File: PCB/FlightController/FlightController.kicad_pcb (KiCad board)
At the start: 2 copper layers, 101.6 x 101.6 mm, 14 parts, among them J2 BATT IN, J3 BATT OUT, J4 BATT Reg IC, J5 Pump, J7 HallCircuit, Q1 P_CHANNEL, U1 XIAO-nRF52840-DIP, U2 RFM95W

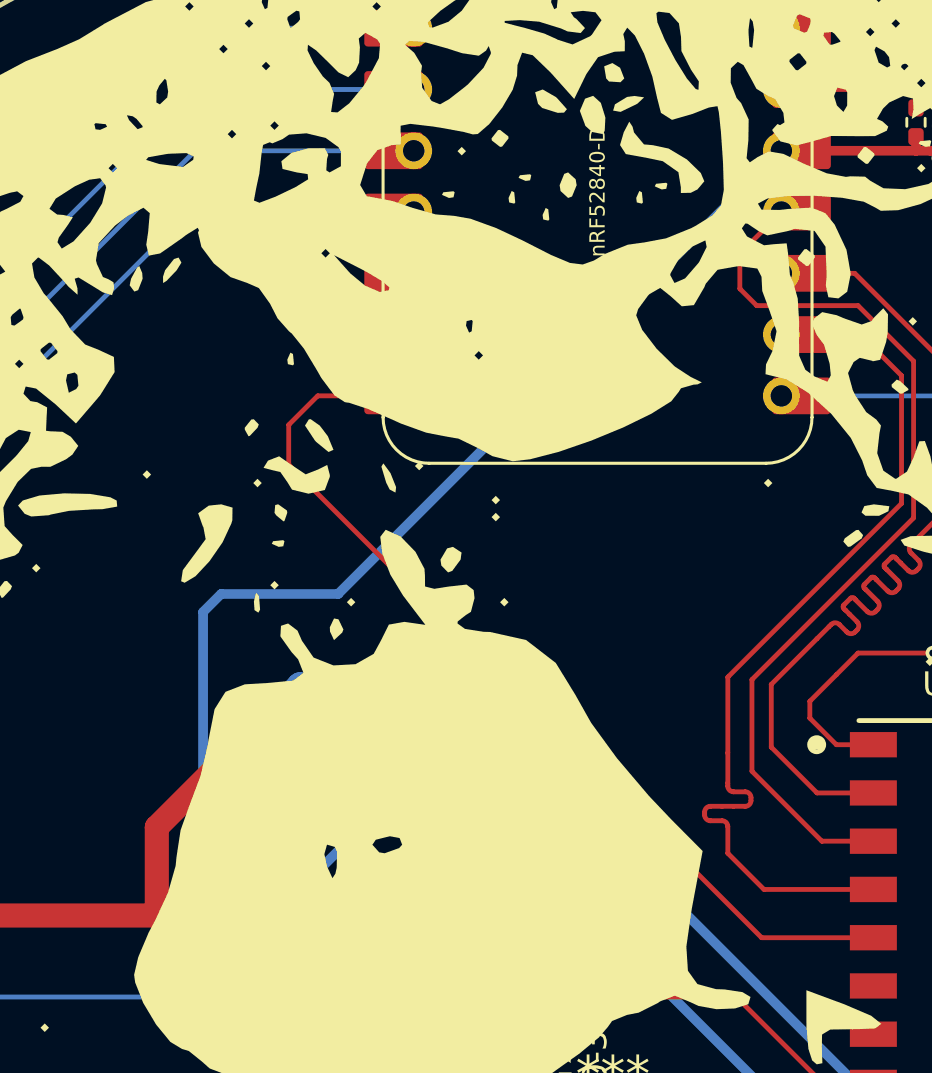
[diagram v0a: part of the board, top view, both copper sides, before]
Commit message: All boards should be finished. ACC otw, and an earlier version of the main board otw
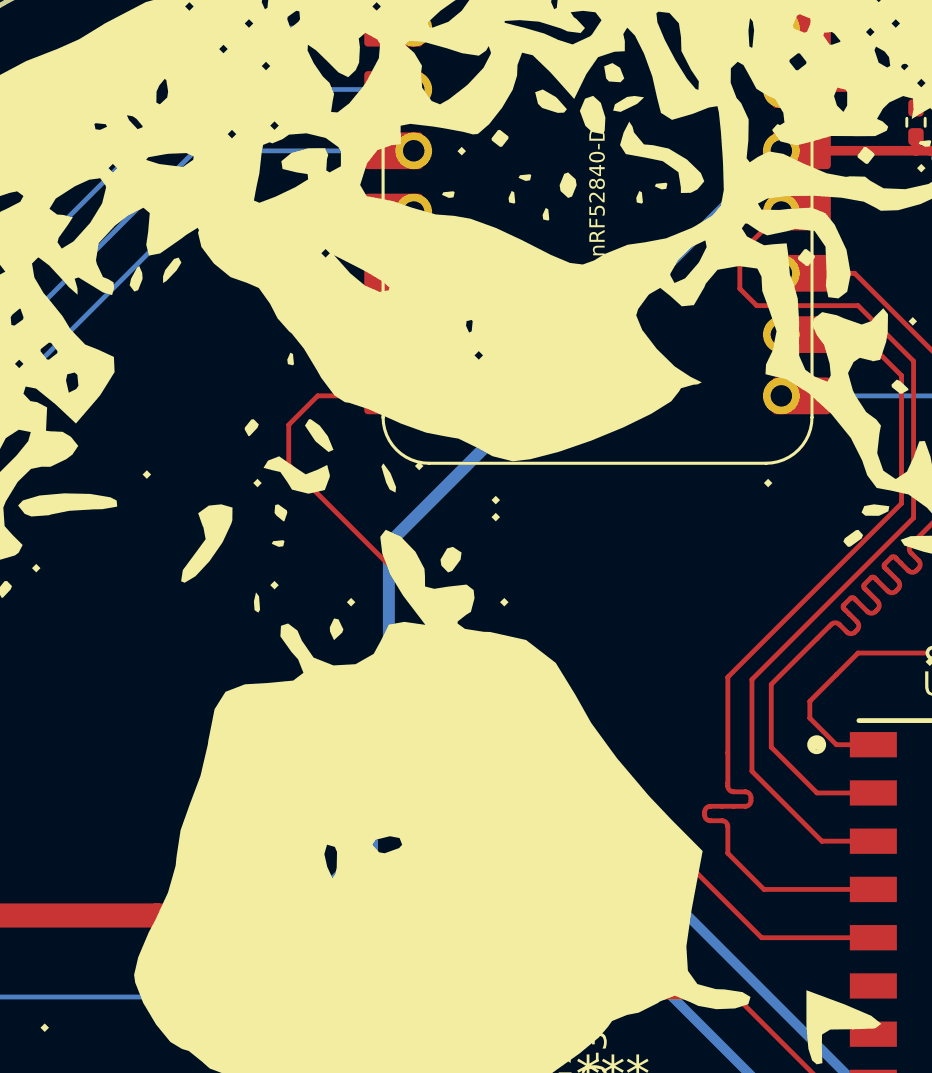
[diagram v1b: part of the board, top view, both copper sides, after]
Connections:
- Q1 pad 2: SWVOUT -> RAWSWPOWER
- Q1 pad 3: RAWSWPOWER -> SWVOUT
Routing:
- net SWVOUT: track 51.6 -> 31.6 mm
- net RAWSWPOWER: track 88.7 -> 83.0 mm
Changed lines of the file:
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@@
 			(size 0.8636 1.6002)
 			(layers "B.Cu" "B.Mask" "B.Paste")
-			(net 24 "SWVOUT")
+			(net 23 "RAWSWPOWER")
 			(pinfunction "2")
 			(pintype "unspecified")
@@
 			(size 0.8636 1.6002)
 			(layers "B.Cu" "B.Mask" "B.Paste")
-			(net 23 "RAWSWPOWER")
+			(net 24 "SWVOUT")
 			(pinfunction "3")
 			(pintype "unspecified")
@@
 	)
 	(segment
-		(start 122.83 79.42)
-		(end 122.83 83.08)
-		(width 1)
-		(layer "F.Cu")
-		(net 23)
-	)
-	(segment
 		(start 170.296051 110.203949)
 		(end 149.953949 110.203949)
@@
 	)
 	(segment
-		(start 127.75 74.5)
-		(end 122.83 79.42)
+		(start 129.1 83.1)
+		(end 129.08 83.08)
 		(width 1)
 		(layer "F.Cu")
 		(net 23)
 	)
+	(segment
+		(start 129.08 83.08)
+		(end 122.83 83.08)
+		(width 1)
+		(layer "F.Cu")
+		(net 23)
+	)
 	(via
-		(at 127.75 74.5)
+		(at 129.1 83.1)
 		(size 0.6)
 		(drill 0.3)
@@
 	)
 	(segment
-		(start 128.75 73.5)
-		(end 127.875 74.375)
+		(start 131.5 78.25)
+		(end 131.5 80.7)
 		(width 1)
 		(layer "B.Cu")
@@
 	)
 	(segment
-		(start 131.5 73.5)
-		(end 128.75 73.5)
+		(start 131.5 80.7)
+		(end 129.1 83.1)
 		(width 1)
 		(layer "B.Cu")
@@
 	)
 	(segment
-		(start 127.875 74.375)
-		(end 127.75 74.5)
-		(width 1)
-		(layer "B.Cu")
-		(net 23)
-	)
-	(segment
 		(start 132.450001 76.239)
-		(end 132.450001 74.450001)
-		(width 1)
-		(layer "B.Cu")
-		(net 23)
-	)
-	(segment
-		(start 132.450001 74.450001)
-		(end 131.5 73.5)
-		(width 1)
-		(layer "B.Cu")
-		(net 23)
-	)
-	(segment
-		(start 125.5 69.75)
-		(end 130.35 69.75)
-		(width 0.4)
+		(end 132.450001 67.649999)
+		(width 0.5)
 		(layer "B.Cu")
 		(net 24)
 	)
 	(segment
-		(start 124.75 70.5)
-		(end 125.5 69.75)
-		(width 0.4)
+		(start 132.450001 67.649999)
+		(end 148.72 51.38)
+		(width 0.5)
 		(layer "B.Cu")
 		(net 24)
-	)
-	(segment
-		(start 129 81.75)
-		(end 125.25 81.75)
-		(width 0.4)
-		(layer "B.Cu")
-		(net 24)
-	)
-	(segment
-		(start 131.5 79.25)
-		(end 129 81.75)
-		(width 0.4)
-		(layer "B.Cu")
-		(net 24)
-	)
-	(segment
-		(start 131.5 78.25)
-		(end 131.5 79.25)
-		(width 0.4)
-		(layer "B.Cu")
-		(net 24)
-	)
-	(segment
-		(start 125.25 81.75)
-		(end 124.75 81.25)
-		(width 0.4)
-		(layer "B.Cu")
-		(net 24)
-	)
-	(segment
-		(start 130.35 69.75)
-		(end 148.72 51.38)
-		(width 0.4)
-		(layer "B.Cu")
-		(net 24)
-	)
-	(segment
-		(start 124.75 81.25)
-		(end 124.75 70.5)
-		(width 0.4)
-		(layer "B.Cu")
-		(net 24)
